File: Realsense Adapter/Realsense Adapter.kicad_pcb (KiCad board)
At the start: 2 copper layers, 20.3 x 22.9 mm, 2 parts, among them J1 USB3_B_Micro

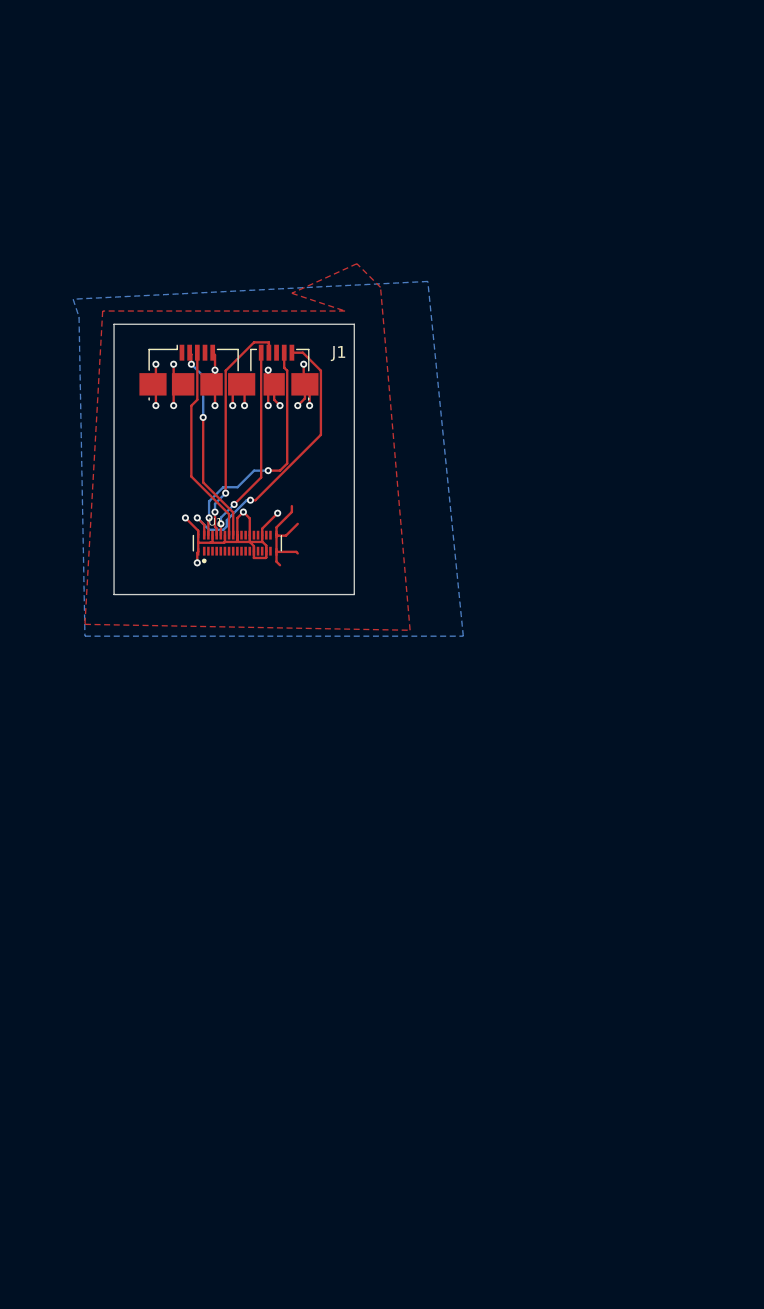
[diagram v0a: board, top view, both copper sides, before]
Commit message: Version v1.0-PROTO of Realsense adapter complete
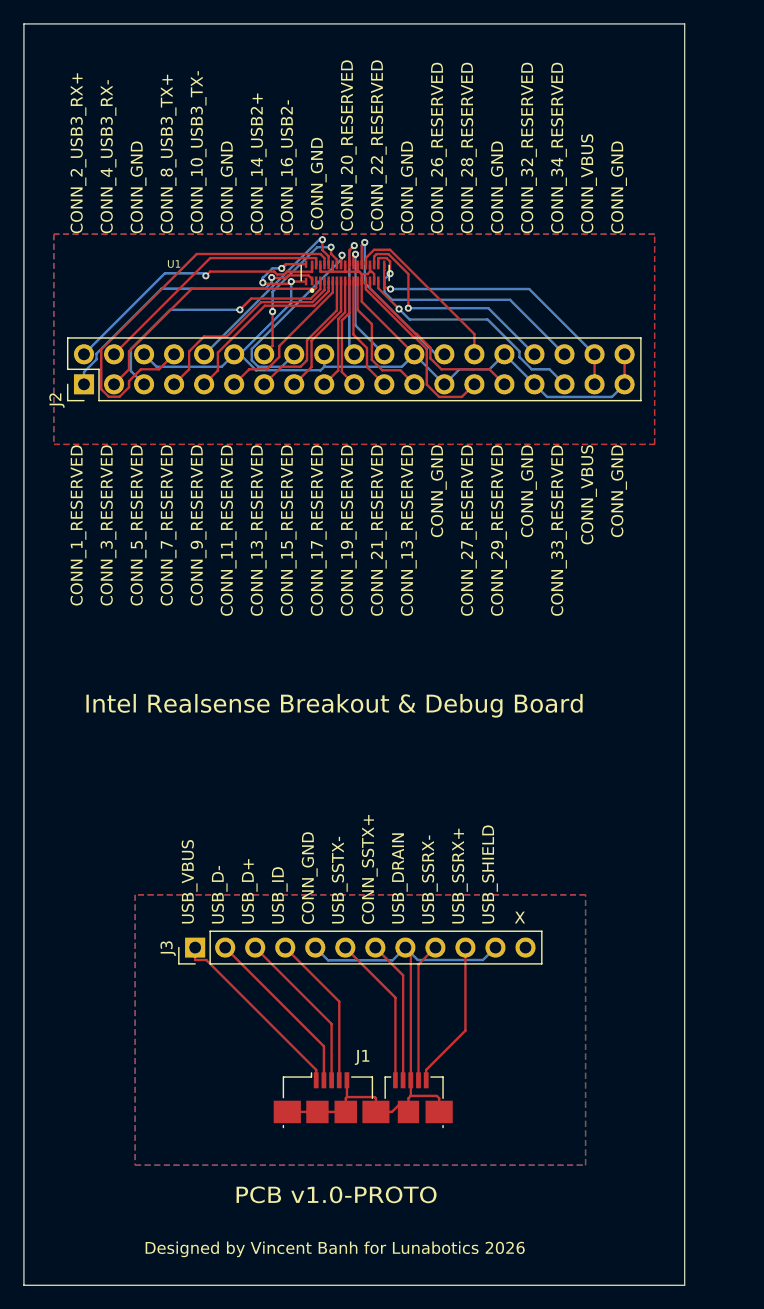
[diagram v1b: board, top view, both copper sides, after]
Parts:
- added G***: LOGO, LOGO, B.Cu at (144.8, 101.6)
- added J2: Conn_02x19_Odd_Even, Connector_PinHeader_2.54mm:PinHeader_2x19_P2.54mm_Vertical, F.Cu at (121.9, 76.2)
- added J3: Conn_01x12_Pin, Connector_PinHeader_2.54mm:PinHeader_1x12_P2.54mm_Vertical, F.Cu at (131.3, 123.8)
- moved J1 62.6 mm to (145.5, 136.5)
- moved U1 24.6 mm to (144.0, 66.8)
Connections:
- J1 pad 1: +5V -> /USB_VBUS
- J1 pad 10: Net-(J1-SSRX+) -> /USB_SSRX+
- J1 pad 11: GND -> /USB_DRAIN
- J1 pad 2: Net-(J1-D-) -> /USB_D-
- J1 pad 3: Net-(J1-D+) -> /USB_D+
- J1 pad 4: unconnected-(J1-ID-Pad4) -> /USB_ID
- J1 pad 5: GND -> /USB_DRAIN
- J1 pad 6: Net-(J1-SSTX-) -> /USB_SSTX-
- J1 pad 7: Net-(J1-SSTX+) -> /USB_SSTX+
- J1 pad 8: unconnected-(J1-DRAIN-Pad8) -> /USB_DRAIN
- J1 pad 9: Net-(J1-SSRX-) -> /USB_SSRX-
- U1 pad 1: unconnected-(U1-Reserved-Pad1) -> /CONN_1_RESERVED
- U1 pad 10: Net-(J1-SSTX-) -> /CONN_10_USB3_TX-
- U1 pad 11: unconnected-(U1-Reserved-Pad11) -> /CONN_11_RESERVED
- U1 pad 12: GND -> /CONN_GND
- U1 pad 13: unconnected-(U1-Reserved-Pad13) -> /CONN_13_RESERVED
- U1 pad 14: Net-(J1-D+) -> /CONN_14_USB2+
- U1 pad 15: unconnected-(U1-Reserved-Pad15) -> /CONN_15_RESERVED
- U1 pad 16: Net-(J1-D-) -> /CONN_16_USB2-
- U1 pad 17: unconnected-(U1-Reserved-Pad17) -> /CONN_17_RESERVED
- U1 pad 18: GND -> /CONN_GND
- U1 pad 19: unconnected-(U1-Reserved-Pad19) -> /CONN_19_RESERVED
- U1 pad 2: Net-(J1-SSRX+) -> /CONN_2_USB3_RX+
- U1 pad 20: unconnected-(U1-Reserved-Pad20) -> /CONN_20_RESERVED
- U1 pad 21: unconnected-(U1-Reserved-Pad21) -> /CONN_21_RESERVED
- U1 pad 22: unconnected-(U1-Reserved-Pad22) -> /CONN_22_RESERVED
- U1 pad 23: unconnected-(U1-Reserved-Pad23) -> /CONN_23_RESERVED
- U1 pad 24: GND -> /CONN_GND
- U1 pad 25: GND -> /CONN_GND
- U1 pad 26: unconnected-(U1-Reserved-Pad26) -> /CONN_26_RESERVED
- U1 pad 27: unconnected-(U1-Reserved-Pad27) -> /CONN_27_RESERVED
- U1 pad 28: unconnected-(U1-Reserved-Pad28) -> /CONN_28_RESERVED
- U1 pad 29: unconnected-(U1-Reserved-Pad29) -> /CONN_29_RESERVED
- U1 pad 3: unconnected-(U1-Reserved-Pad3) -> /CONN_3_RESERVED
- U1 pad 30: GND -> /CONN_GND
- U1 pad 31: GND -> /CONN_GND
- U1 pad 32: unconnected-(U1-Reserved-Pad32) -> /CONN_32_RESERVED
- U1 pad 33: unconnected-(U1-Reserved-Pad33) -> /CONN_33_RESERVED
- U1 pad 34: unconnected-(U1-Reserved-Pad34) -> /CONN_34_RESERVED
- U1 pad 4: Net-(J1-SSRX-) -> /CONN_4_USB3_RX-
- U1 pad 5: unconnected-(U1-Reserved-Pad5) -> /CONN_5_RESERVED
- U1 pad 6: GND -> /CONN_GND
- U1 pad 7: unconnected-(U1-Reserved-Pad7) -> /CONN_7_RESERVED
- U1 pad 8: Net-(J1-SSTX+) -> /CONN_8_USB3_TX+
- U1 pad 9: unconnected-(U1-Reserved-Pad9) -> /CONN_9_RESERVED
- U1 pad S1: GND -> /CONN_GND
- U1 pad S2: +5V -> /CONN_VBUS
- U1 pad S3: GND -> /CONN_GND
- U1 pad S4: +5V -> /CONN_VBUS
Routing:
- net /CONN_GND: track 0.00 -> 86.3 mm, vias 0 -> 3
- net GND: track 52.0 -> 0.00 mm, vias 18 -> 0
- net /USB_DRAIN: track 0.00 -> 49.1 mm
- net /CONN_8_USB3_TX+: track 0.00 -> 34.5 mm
- net Net-(J1-SSRX+): track 24.7 -> 0.00 mm, vias 2 -> 0
- net /CONN_VBUS: track 0.00 -> 24.6 mm, vias 0 -> 1
- net /CONN_1_RESERVED: track 0.00 -> 24.6 mm, vias 0 -> 1
- net /CONN_2_USB3_RX+: track 0.00 -> 23.1 mm, vias 0 -> 1
- net /CONN_5_RESERVED: track 0.00 -> 22.3 mm, vias 0 -> 1
- net /CONN_3_RESERVED: track 0.00 -> 21.9 mm
- net /CONN_34_RESERVED: track 0.00 -> 21.9 mm, vias 0 -> 1
- net /CONN_4_USB3_RX-: track 0.00 -> 21.0 mm
- net Net-(J1-SSRX-): track 20.3 -> 0.00 mm, vias 2 -> 0
- net /CONN_33_RESERVED: track 0.00 -> 20.0 mm, vias 0 -> 1
- net Net-(J1-SSTX+): track 19.9 -> 0.00 mm, vias 2 -> 0
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- added copper zone on B.Cu, net /CONN_GND
- added copper zone on F.Cu, net /CONN_GND
- added copper zone on B.Cu, net /USB_DRAIN
- added copper zone on F.Cu, net /USB_DRAIN
- removed copper zone on F.Cu, net +5V
- removed copper zone on B.Cu, net GND
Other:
- board size 20.3 x 22.9 mm -> 55.9 x 106.7 mm
- board text added: "CONN_10_USB3_TX-"
- board text added: "CONN_11_RESERVED"
- board text added: "CONN_13_RESERVED"
- board text added: "CONN_14_USB2+"
- board text added: "CONN_15_RESERVED"
- board text added: "CONN_16_USB2-"
- board text added: "CONN_17_RESERVED"
- board text added: "CONN_19_RESERVED"
- board text added: "CONN_1_RESERVED"
- board text added: "CONN_20_RESERVED"
- board text added: "CONN_21_RESERVED"
- board text added: "CONN_22_RESERVED"
- board text added: "CONN_26_RESERVED"
- board text added: "CONN_27_RESERVED"
- board text added: "CONN_28_RESERVED"
- board text added: "CONN_29_RESERVED"
- board text added: "CONN_2_USB3_RX+"
- board text added: "CONN_32_RESERVED"
- board text added: "CONN_33_RESERVED"
- board text added: "CONN_34_RESERVED"
- board text added: "CONN_3_RESERVED"
- board text added: "CONN_4_USB3_RX-"
- board text added: "CONN_5_RESERVED"
- board text added: "CONN_7_RESERVED"
- board text added: "CONN_8_USB3_TX+"
- board text added: "CONN_9_RESERVED"
- board text added: "CONN_GND"
- board text added: "CONN_SSTX+"
- board text added: "CONN_VBUS"
- board text added: "Designed by Vincent Banh for Lunabotics 2026"
- board text added: "Intel Realsense Breakout & Debug Board"
- board text added: "PCB v1.0-PROTO"
- board text added: "USB_D+"
- board text added: "USB_D-"
- board text added: "USB_DRAIN"
- board text added: "USB_ID"
- board text added: "USB_SHIELD"
- board text added: "USB_SSRX+"
- board text added: "USB_SSRX-"
- board text added: "USB_SSTX-"
- board text added: "USB_VBUS"
- board text added: "Version numbering order Major.minor - tag (if needed) Examples: - v1.0-PROTO (Prototype for version 1.0 of the design) - v1.0-FINAL (Final production design for version 1.0) - v1.1 (Minor update to v1.0 - maybe a wiring mistake is fixed, or a footprint has changed) - v2.0-PROTO (Major overhaul - new features added or removed)"
- board text added: "X"
